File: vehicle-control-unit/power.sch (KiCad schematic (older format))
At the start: 9 parts, among them J13 Conn_01x02_Male, SW1 SW_SPST, U4 MIC29502WT

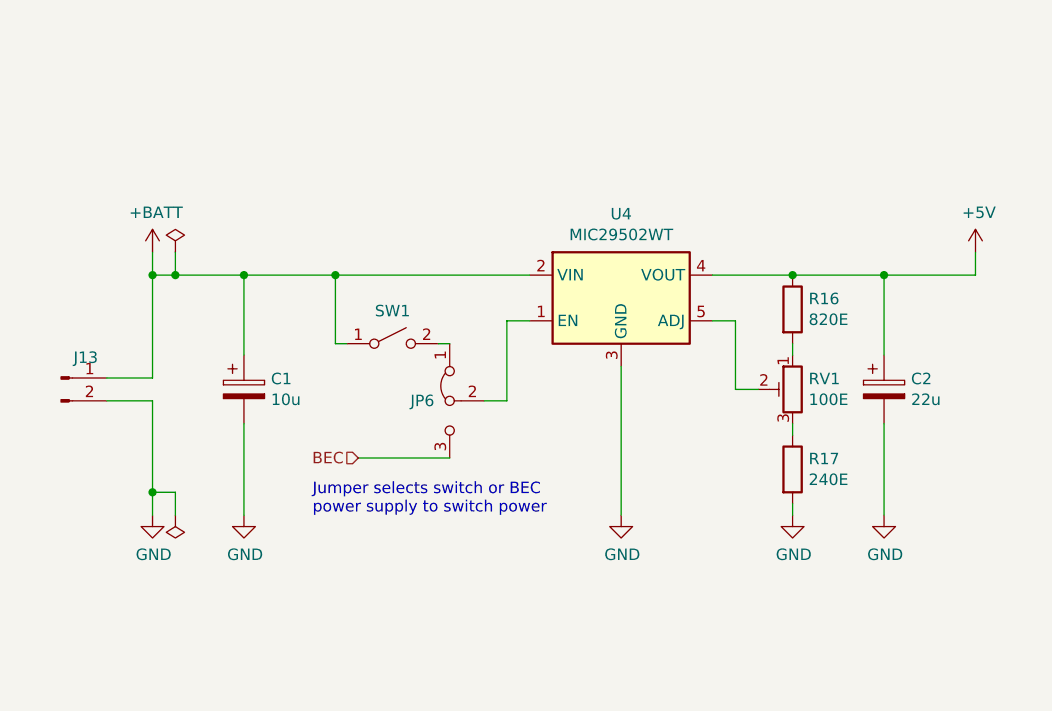
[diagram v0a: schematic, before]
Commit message: Review schematics
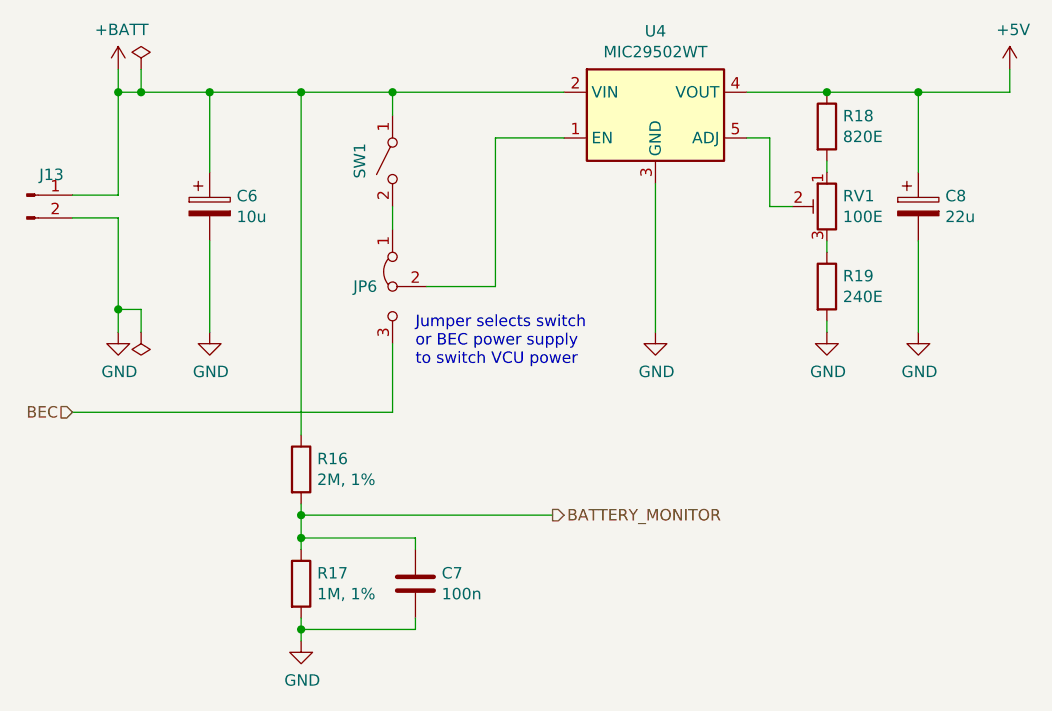
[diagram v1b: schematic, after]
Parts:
- added C7: 100n, symbol Device:C
- added R16: 2M, 1%, symbol Device:R
- added R17: 1M, 1%, symbol Device:R
- renumbered C1 to C6, C2 to C8, R16 to R18, R17 to R19
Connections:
- net +BATT: now also R16.1
- net GND: now also C7.2, R17.2
- new net BATTERY_MONITOR: C7.1, R16.2, R17.1
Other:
- note added: "Jumper selects switch\nor BEC power supply\nto switch VCU power"
- note removed: "Jumper selects switch or BEC\npower supply to switch power"
- moved on the sheet: C6, C8, J13, JP6, R18, R19, RV1, SW1, U4
